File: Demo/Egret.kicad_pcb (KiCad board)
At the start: 2 copper layers, 10 x 7.2 mm, 34 parts, among them J1 Conn_01x08_Male, J2 Micro_SD_Card, J3 2388749-1, Q1 S8050, Q2 S8050, U1 MPU6050, U2 LP2992IM5-3.3, U3 BH1750FVI-TR, U4 WS2812B-B, U5 ESP32-PICO-D4, U6 AN2051, U7 CP2102N-A01-GQFN28

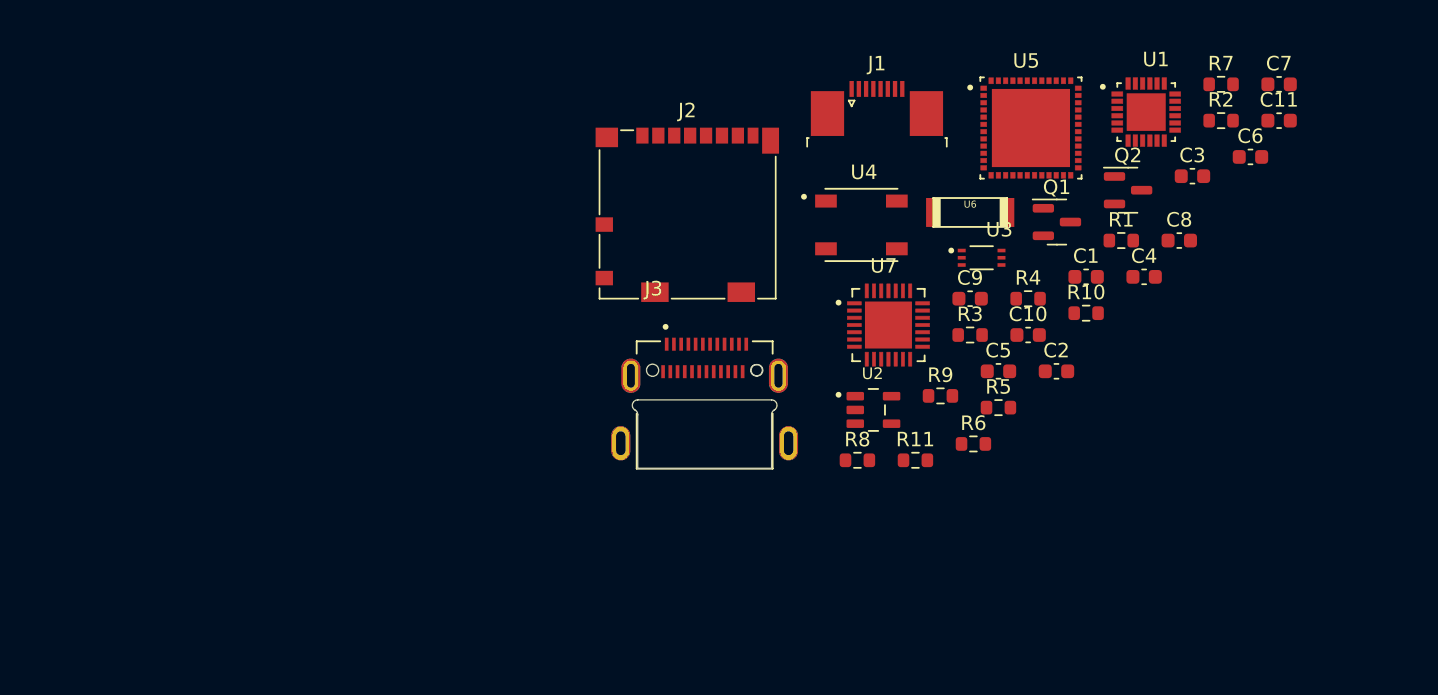
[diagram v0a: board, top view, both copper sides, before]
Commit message: update
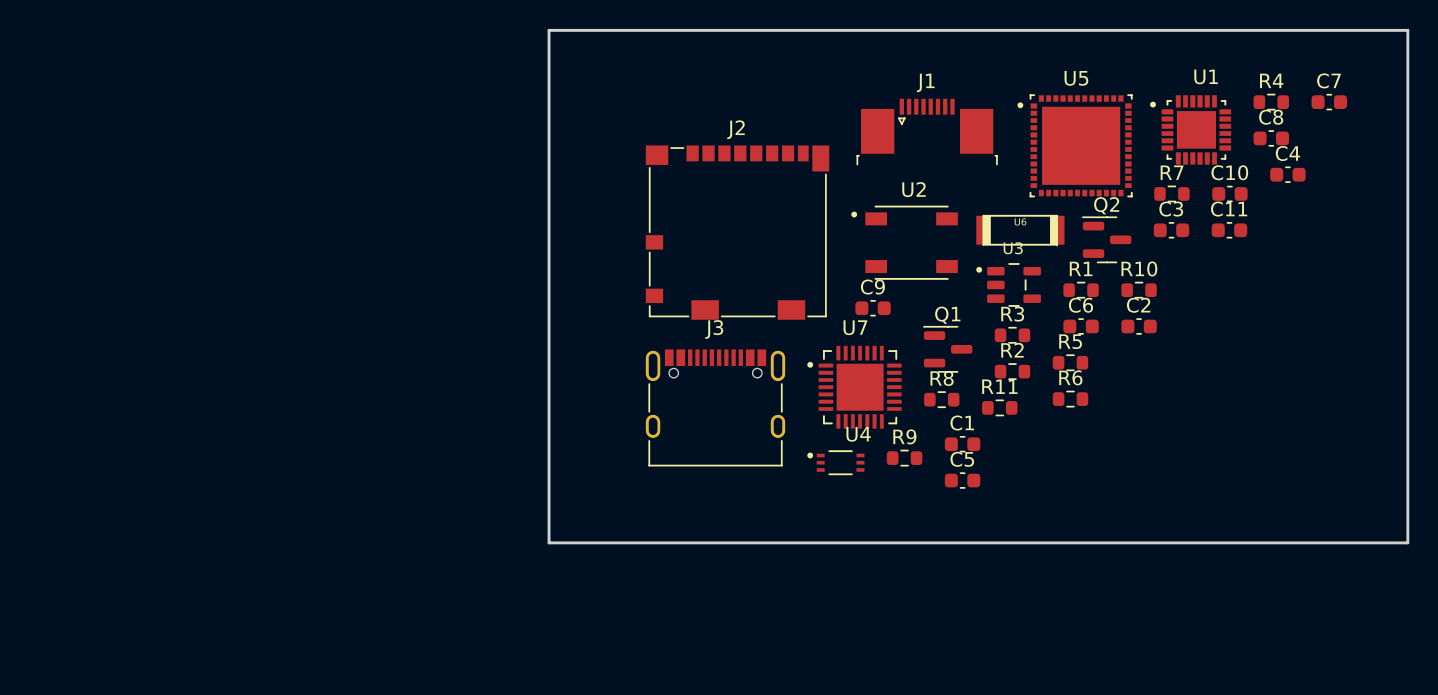
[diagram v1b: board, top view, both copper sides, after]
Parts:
- C6: value 0.1uF -> 10uF
- C7: value 10uF -> 10nF
- C8: value 10nF -> 0.1uF
- J3: value 2388749-1 -> USB_C_Receptacle; footprint 2388749-1:TE_2388749-1 -> Connector_USB:USB_C_Receptacle_XKB_U262-16XN-4BVC11
- U2: value LP2992IM5-3.3 -> WS2812B-B; footprint LP2992IM5-3:SOT95P280X145-5N -> WS2812B-B:LED_WS2812B-B
- U3: value BH1750FVI-TR -> LP2992IM5-3.3; footprint BH1750FVI-TR:XDCR_BH1750FVI-TR -> LP2992IM5-3:SOT95P280X145-5N
- U4: value WS2812B-B -> BH1750FVI-TR; footprint WS2812B-B:LED_WS2812B-B -> BH1750FVI-TR:XDCR_BH1750FVI-TR
- moved R2 22.6 mm to (172.3, 93.6)
- moved R4 21.6 mm to (190.2, 75.0)
- moved C10 17.0 mm to (187.4, 81.3)
- moved C6 16.6 mm to (177.1, 90.5)
- moved U4 16.5 mm to (160.5, 99.9)
- moved C1 14.4 mm to (168.9, 98.6)
- moved C4 12.2 mm to (191.4, 80.0)
- moved U2 11.9 mm to (165.4, 84.7)
- moved Q1 11.6 mm to (167.9, 92.0)
- moved C8 9.50 mm to (190.2, 77.5)
- moved C11 8.32 mm to (187.3, 83.8)
- moved R7 8.31 mm to (183.4, 81.3)
- moved C5 7.95 mm to (168.9, 101.1)
- moved R6 7.39 mm to (176.3, 95.5)
- moved R8 7.18 mm to (167.4, 95.5)
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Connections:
- C5 pad 1: +3V3 -> GND
- C5 pad 2: GND -> +3V3
- C7 pad 1: GND -> +3V3
- C7 pad 2: +3V3 -> GND
- U2 pad 2: GND -> unconnected-(U2-Pad2)
- U2 pad 3: +5V -> GND
- U2 pad 4: Net-(C1-Pad1) -> /GPIO27
- U3 pad 1: +3V3 -> +5V
- U3 pad 3: GND -> +5V
- U3 pad 4: /BH_SDA -> Net-(C1-Pad1)
- U3 pad 5: Net-(R1-Pad1) -> +3V3
- U4 pad 1: +5V -> +3V3
- U4 pad 2: unconnected-(U4-Pad2) -> GND
- U4 pad 4: /GPIO27 -> /BH_SDA
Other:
- board size 10 x 7.2 mm -> 59.4 x 35.4 mm

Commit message: update
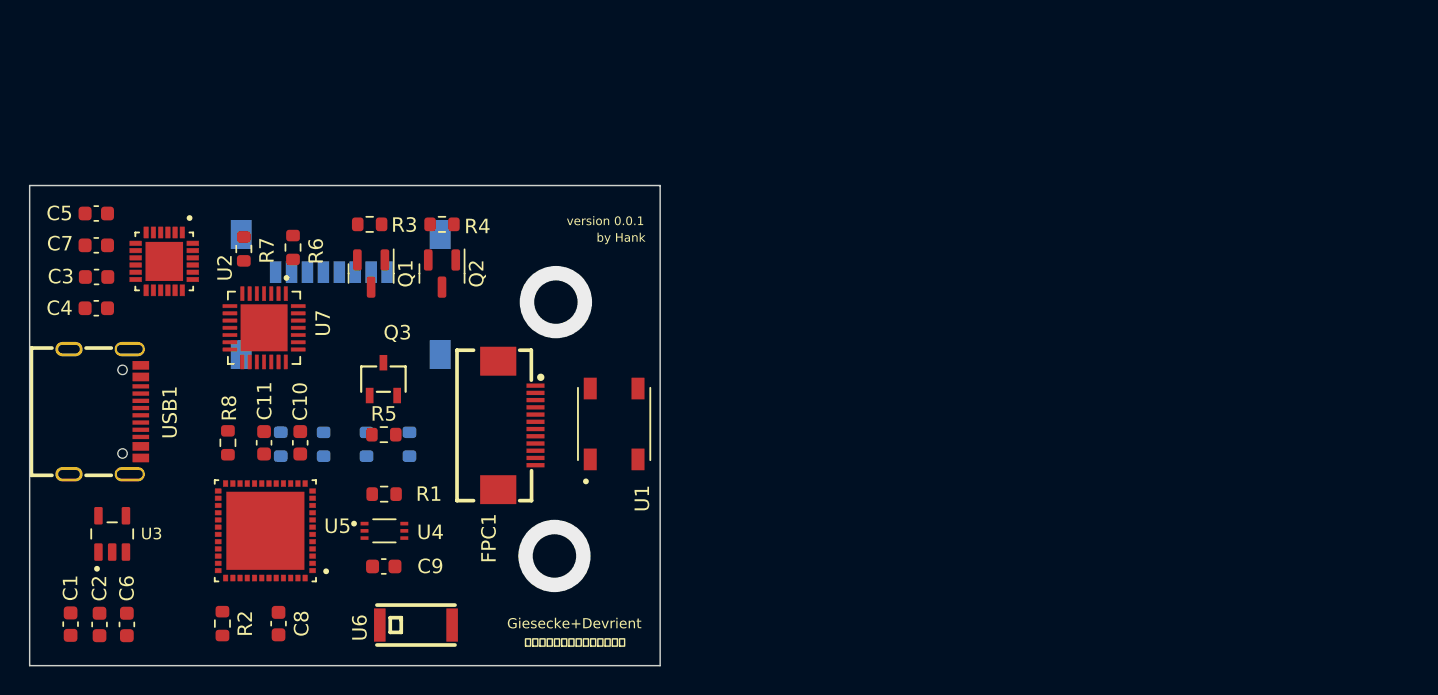
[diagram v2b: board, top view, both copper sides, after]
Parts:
- removed J2: Micro_SD_Card, Connector_Card:microSD_HC_Molex_104031-0811
- removed J3: USB_C_Receptacle, Connector_USB:USB_C_Receptacle_XKB_U262-16XN-4BVC11
- added FPC1: FPC-05F-12PH20, kicad_lceda:FPC-SMD_12P-P0.50_FPC-05F-12PH20, F.Cu at (138.1, 97.3)
- added G***: LOGO, G+D:logo, B.Cu at (127.2, 97.5)
- added Q3: AO3415AL, kicad_lceda:SOT-23-3_L2.9-W1.6-P1.90-LS2.9-BL, F.Cu at (128.8, 94.1)
- added R12: 10k, Resistor_SMD:R_0603_1608Metric, B.Cu at (130.7, 98.6)
- added USB1: TYPEC-304J-BCP16, kicad_lceda:USB-C-SMD_TYPEC-304J-BCP16, F.Cu at (109.6, 96.3)
- C4: value 2.2nF -> 0.1uF
- C5: value 0.1uF -> 2.2nF
- J1: value Conn_01x08_Male -> Micro_SD_Card; footprint Connector_FFC-FPC:TE_0-1734839-8_1x08-1MP_P0.5mm_Horizontal -> Connector_Card:microSD_HC_Wuerth_693072010801; moved to B.Cu
- R10, R11, R9: moved to B.Cu
- R5: value 200R -> 1k
- R6: value 10k -> 200R
- R7: value 0 -> 10k
- R8: value 10k -> 0
- U1: value MPU6050 -> WS2812B-B; footprint MPU6050:IC_MPU6050 -> WS2812B-B:LED_WS2812B-B
- U2: value WS2812B-B -> MPU6050; footprint WS2812B-B:LED_WS2812B-B -> MPU6050:IC_MPU6050
- U6: value AN2051 -> AN2051-245_2.4G全向天线; footprint AN2051:AN2051 -> kicad_lceda:ANT-SMD_L5.0-W2.0
- moved C7 85.8 mm to (109.0, 84.8)
- moved C4 82.9 mm to (109.0, 89.2)
- moved C8 76.4 mm to (121.6, 111.0), turned to 90 degrees
- moved C2 74.8 mm to (109.2, 111.1), turned to 90 degrees
- moved C3 74.4 mm to (109.0, 87.0)
- moved C6 69.1 mm to (111.1, 111.1), turned to 90 degrees
- moved C11 68.3 mm to (120.6, 98.5), turned to 90 degrees
- moved C10 66.5 mm to (123.1, 98.5), turned to 90 degrees
- moved U3 64.7 mm to (110.1, 104.8), turned to 90 degrees
- moved R7 64.3 mm to (119.2, 85.1), turned to -90 degrees
- moved C1 62.9 mm to (107.2, 111.0), turned to -90 degrees
- moved C5 62.7 mm to (109.0, 82.7)
- moved U5 62.4 mm to (120.7, 104.6), turned to 180 degrees
- moved R4 57.9 mm to (132.9, 83.4)
- moved R10 57.4 mm to (124.7, 98.6), turned to -90 degrees
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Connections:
- C2 pad 1: +3V3 -> GND
- C2 pad 2: GND -> +3V3
- C3 pad 1: Net-(C3-Pad1) -> +3V3
- C5 pad 1: GND -> Net-(C5-Pad1)
- C5 pad 2: +3V3 -> GND
- C8 pad 1: +3V3 -> /EN
- C9 pad 1: /EN -> +3V3
- J1 pad 1: /GPIO5 -> unconnected-(J1-Pad1)
- J1 pad 2: /GPIO4 -> /GPIO15/SD_CS
- J1 pad 3: /GPIO23 -> /GPIO13/SD_MOSI
- J1 pad 4: /GPIO18 -> +3V3
- J1 pad 5: /DC -> /GPIO14/SD_CLK
- J1 pad 7: +3V3 -> /GPIO26/SD_MISO
- J1 pad 8: +5V -> unconnected-(J1-Pad8)
- R10 pad 1: /GPIO14 -> /GPIO13/SD_MOSI
- R11 pad 1: /GPIO15 -> /GPIO14/SD_CLK
- R5 pad 1: /CP_Tx -> Net-(Q3-Pad1)
- R5 pad 2: Net-(R5-Pad2) -> /GPIO5/LCD_BL
- R6 pad 1: +5V -> /CP_Tx
- R7 pad 1: +3V3 -> +5V
- R7 pad 2: /3V3A -> Net-(R7-Pad2)
- R8 pad 1: /GPIO26 -> +3V3
- R8 pad 2: +3V3 -> /3V3A
- R9 pad 1: /GPIO13 -> /GPIO26/SD_MISO
- U1 pad 1: GND -> +5V
- U1 pad 3: unconnected-(U1-Pad3) -> GND
- U1 pad 4: unconnected-(U1-Pad4) -> /GPIO27/RGB_LED
- U2 pad 1: +5V -> GND
- U2 pad 3: GND -> unconnected-(U2-Pad3)
- U2 pad 4: /GPIO27 -> unconnected-(U2-Pad4)
- U4 pad 4: /BH_SDA -> /GPIO32/MPU_SDA/BH_SDA
- U4 pad 6: /BH_SCL -> /GPIO33/MPU_SCL/BH_SCL
- U5 pad 10: /GPIO34 -> unconnected-(U5-Pad10)
- U5 pad 11: /GPIO35 -> unconnected-(U5-Pad11)
- U5 pad 12: /BH_SDA -> /GPIO32/MPU_SDA/BH_SDA
- U5 pad 13: /BH_SCL -> /GPIO33/MPU_SCL/BH_SCL
- U5 pad 15: /GPIO26 -> /GPIO26/SD_MISO
- U5 pad 16: /GPIO27 -> /GPIO27/RGB_LED
- U5 pad 17: /GPIO14 -> /GPIO14/SD_CLK
- U5 pad 20: /GPIO13 -> /GPIO13/SD_MOSI
- U5 pad 21: /GPIO15 -> /GPIO15/SD_CS
- U5 pad 22: /DC -> /GPIO2/DC
- U5 pad 24: /GPIO4 -> /GPIO4/RES
- U5 pad 34: /GPIO5 -> /GPIO5/LCD_BL
- U5 pad 35: /GPIO18 -> /GPIO18/SCK
- U5 pad 36: /GPIO23 -> /GPIO23/MOSI
- U5 pad 5: /SENSOR_VP -> unconnected-(U5-Pad5)
- U5 pad 6: /GPIO37 -> unconnected-(U5-Pad6)
- U5 pad 7: /GPIO38 -> unconnected-(U5-Pad7)
- U5 pad 8: /SENSOR_VN -> unconnected-(U5-Pad8)
- U7 pad 26: Net-(R5-Pad2) -> Net-(R6-Pad2)
- U7 pad 9: Net-(R6-Pad2) -> Net-(R7-Pad2)
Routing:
- net (no net): vias 0 -> 2
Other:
- board size 59.4 x 35.4 mm -> 43.6 x 33.2 mm
- board text added: "Giesecke+Devrient"
- board text added: "by Hank"
- board text added: "version 0.0.1"
- board text added: "捷德（中国）信息科技有限公司"
